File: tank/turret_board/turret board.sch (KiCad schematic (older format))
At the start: 29 parts, among them J1 Conn_01x06, J2 Conn_01x06, Q1 Q_NPN_BCE, Q2 Q_NPN_BCE, U1 LM317T, U2 pixart_ir, Y1 Crystal_4pin

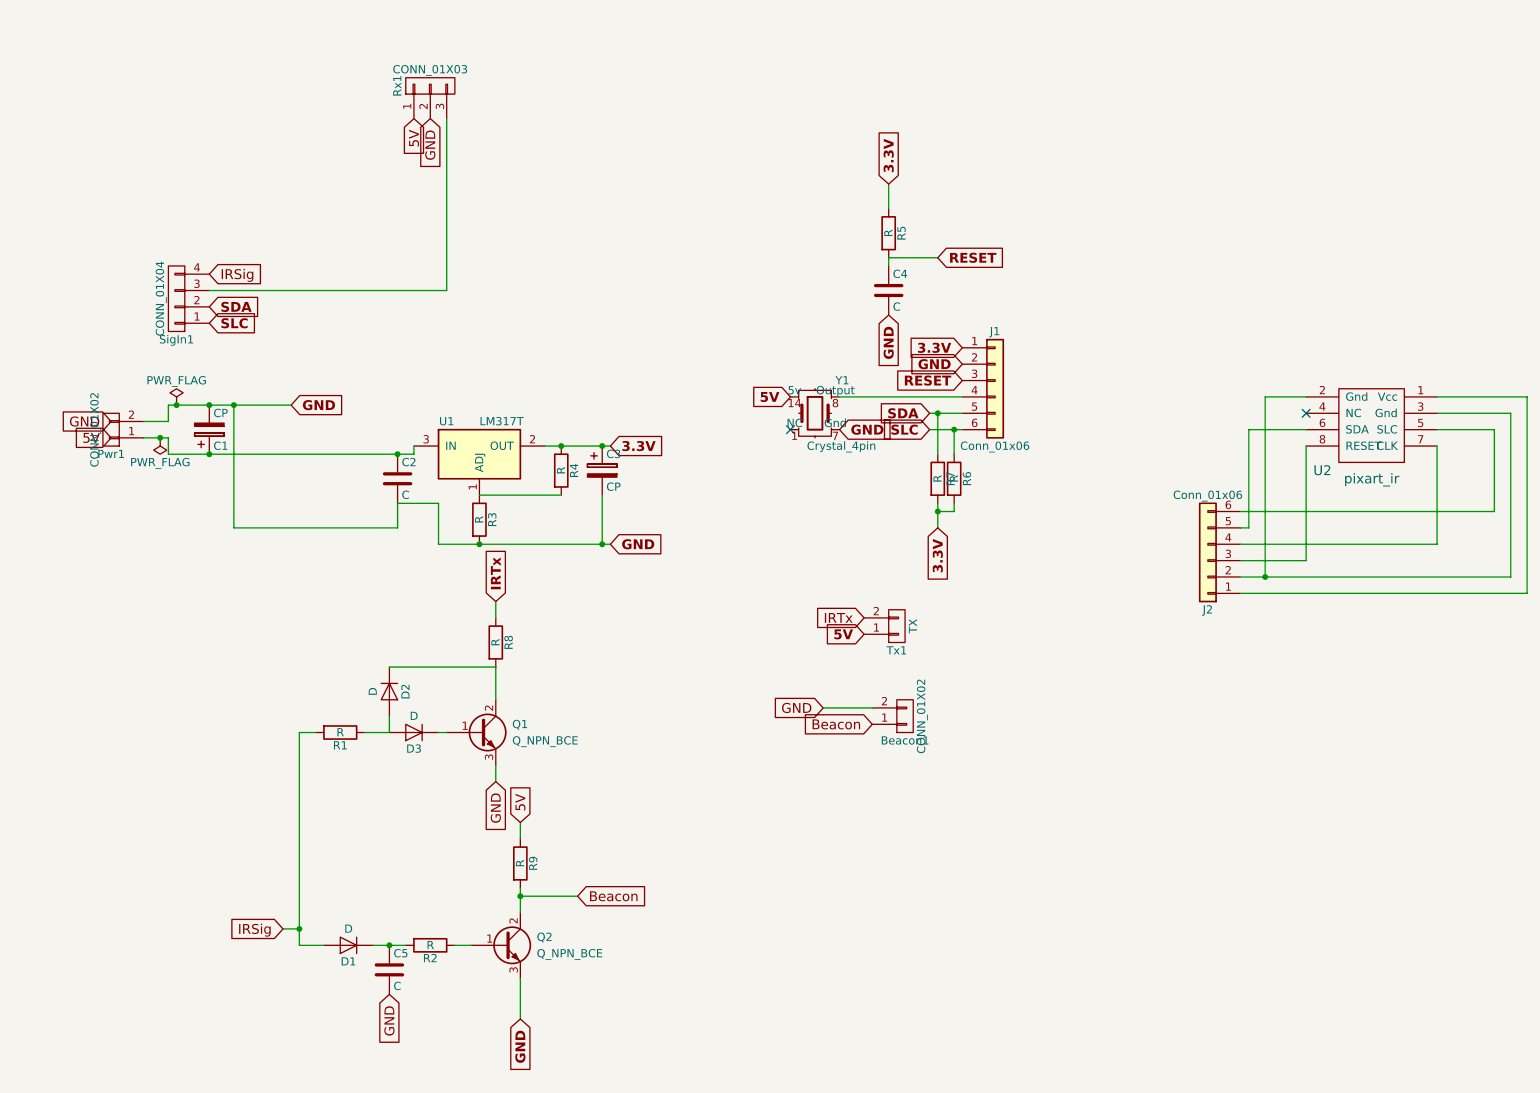
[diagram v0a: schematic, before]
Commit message: interim
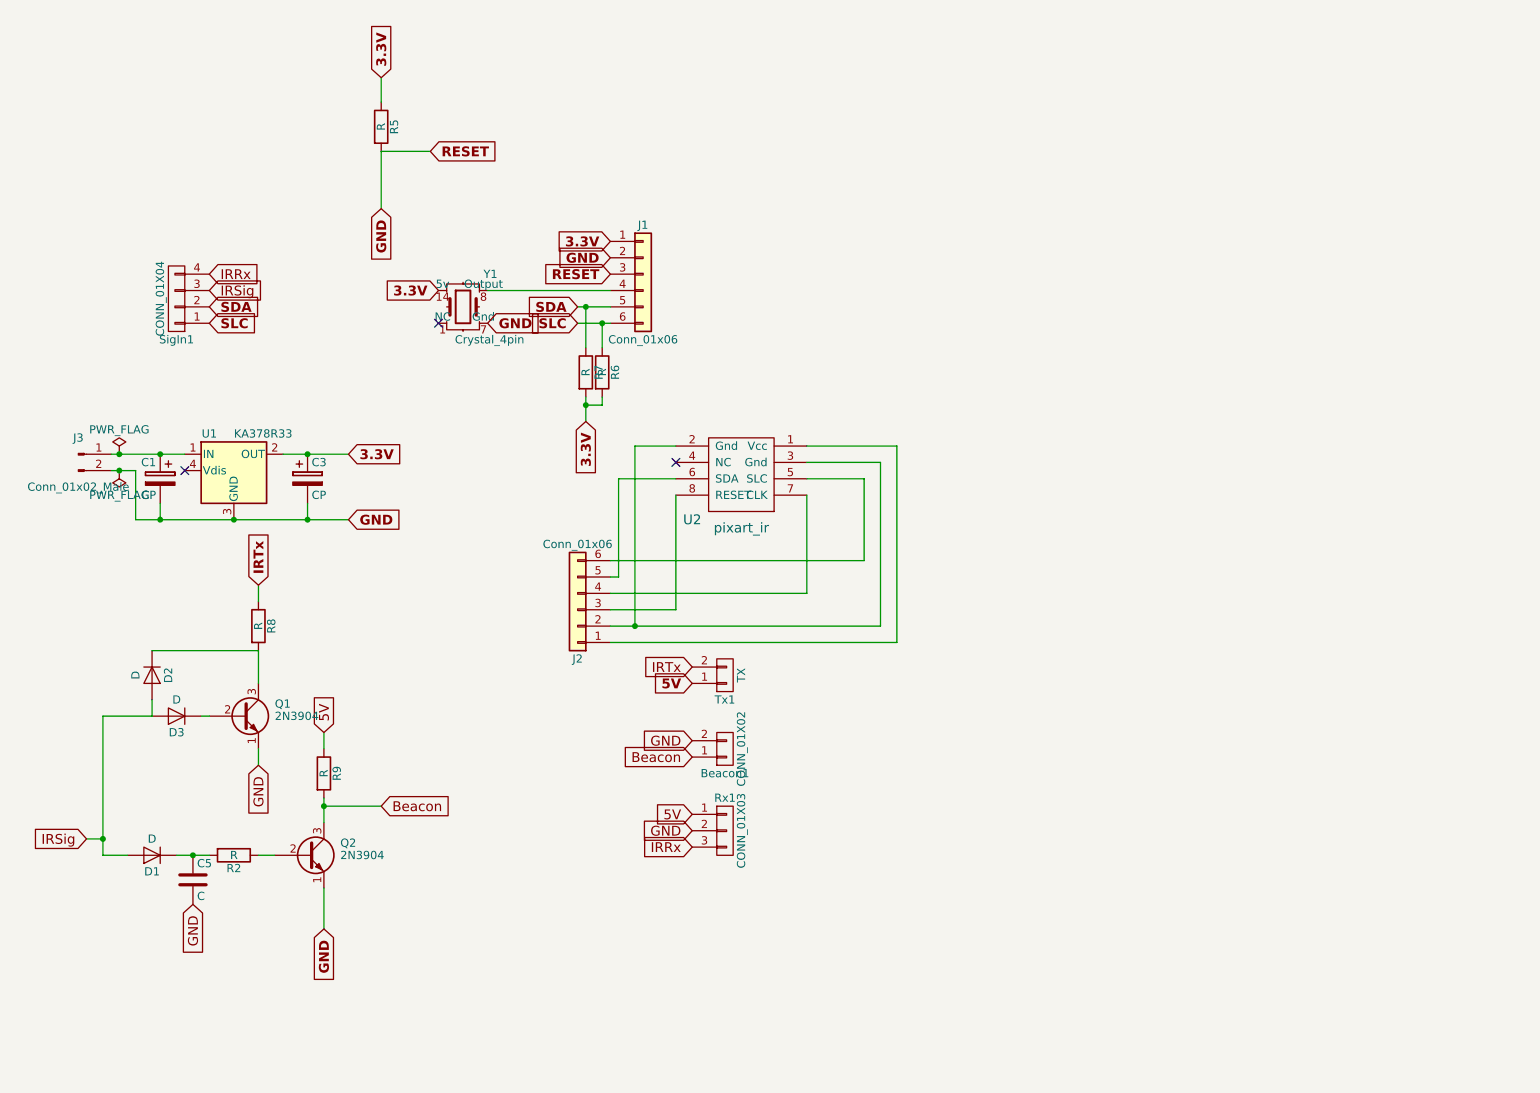
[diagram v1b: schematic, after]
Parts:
- removed C2, C4: C, Capacitors_THT:C_Disc_D3.0mm_W1.6mm_P2.50mm, symbol C
- removed Pwr1: CONN_01X02, JST:JST_EH_B02B-EH-A_02x2.50mm_Straight, symbol CONN_01X02
- removed Q1, Q2: Q_NPN_BCE, Transistors_OldSowjetAera:OldSowjetaera_Transistor_Type-I_SmallPads, symbol Q_NPN_BCE
- removed R1, R3, R4: R, Resistors_THT:R_Axial_DIN0207_L6.3mm_D2.5mm_P7.62mm_Horizontal, symbol R
- removed U1: LM317T, Tank:LM317T, symbol LM317T
- added J3: Conn_01x02_Male, JST:JST_EH_B02B-EH-A_02x2.50mm_Straight, symbol Conn_01x02_Male
- added Q1, Q2: 2N3904, TO_SOT_Packages_THT:TO-92_Inline_Narrow_Oval, symbol 2N3904
- added U1: KA378R33, TO_SOT_Packages_THT:TO-220-4_Vertical, symbol KA378R33
- J1, J2: footprint Connectors_JAE:JAE_LY20-06P-2T_2x03x2.00mm_Straight -> Pin_Headers:Pin_Header_Straight_2x03_Pitch2.54mm
- U2: footprint Tank:pixart_ir -> modules:pixart_ir
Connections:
- net RESET is gone; now on net GND: J1.3 (Pin_3), R5.2
- net 3.3V: now also Y1.14 (5v), U1.2 (OUT)
- net 5V: no longer Y1.14 (5v)
- net Beacon: now also Q2.3 (C)
- net GND: now also J3.2 (Pin_2), Q1.1 (E), Q2.1 (E), U1.3 (GND)
- net IRSig: now also D2.2 (A), D3.2 (A), SigIn1.3 (P3); no longer SigIn1.4 (P4)
- net at C1.1: now also J3.1 (Pin_1), U1.1 (IN)
- net IRRx: now reaches Rx1.3 (P3)
- net IRRx: now also SigIn1.4 (P4); no longer SigIn1.3 (P3)
- net at R2.1: now also Q2.2 (B)
- net at D3.1 (K): now also Q1.2 (B)
- net at D2.1 (K), R8.2: now also Q1.3 (C)
- no-connect marks 2 -> 3
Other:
- moved on the sheet: Beacon1, C1, C3, C5, D1, D2, D3, J1, J2, R2, R5, R6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
